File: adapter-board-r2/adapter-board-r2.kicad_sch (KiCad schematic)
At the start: 47 parts, among them J1 USB_C_Receptacle_USB2.0_14P, J2 Conn_01x02_Socket, J3 Conn_01x04_Socket, J4 Conn_01x07_Pin, Q1 UMH3N, Q2 BSS138W, Q3 BSS138W, U1 ESP32-C3-WROOM-02, U2 USBLC6-2SC6, U3 CH340X, U4 AP2114HA-3.3TRG1, U5 ENS210, U6 LIS2DW12TR, U7 SCD40-D-R2, U8 YSN8900AP3, U9 BMP580

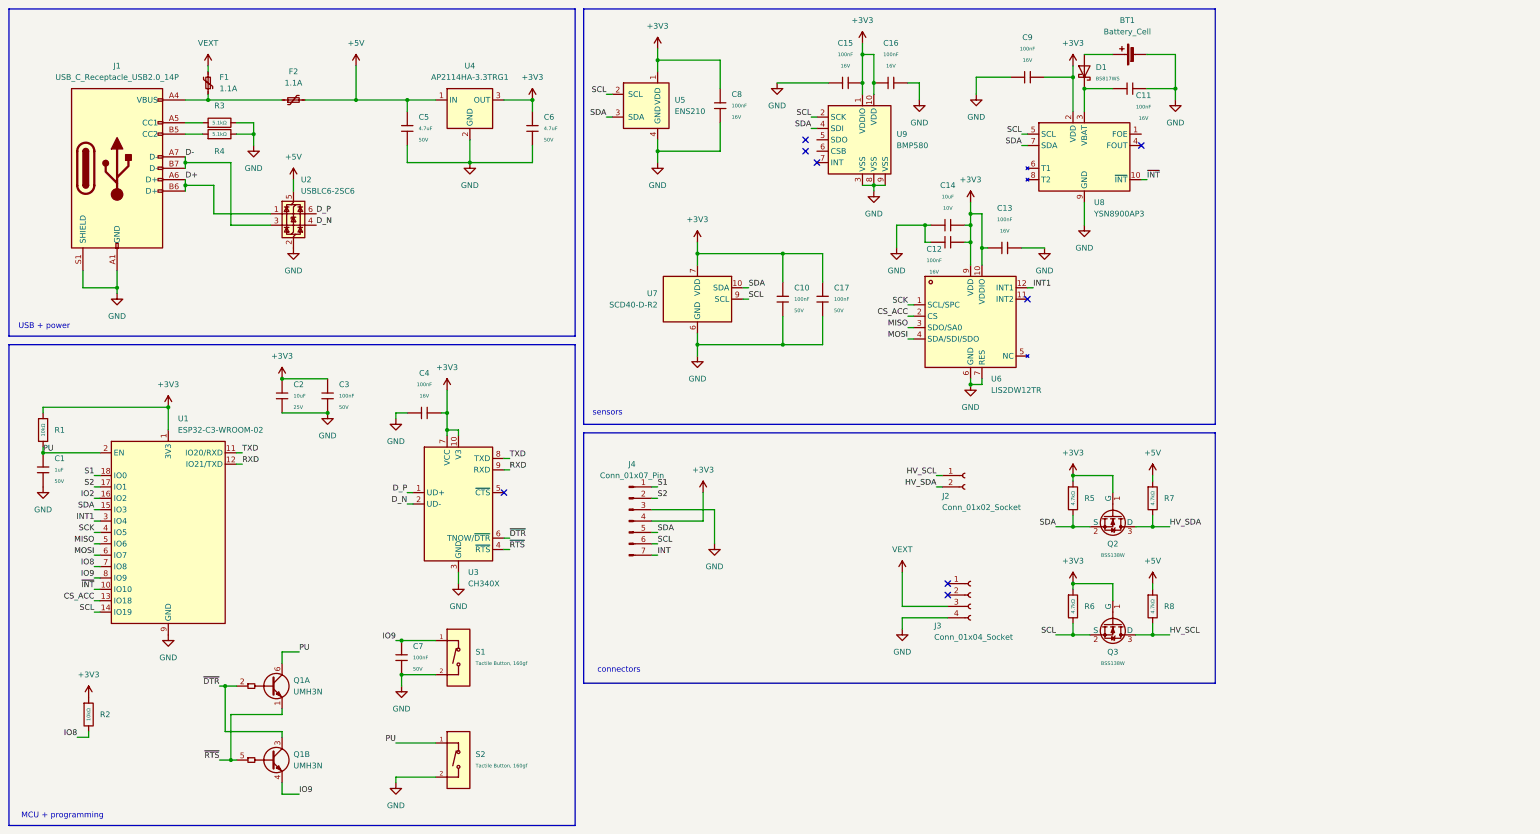
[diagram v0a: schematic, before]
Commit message: feat: updated pcb
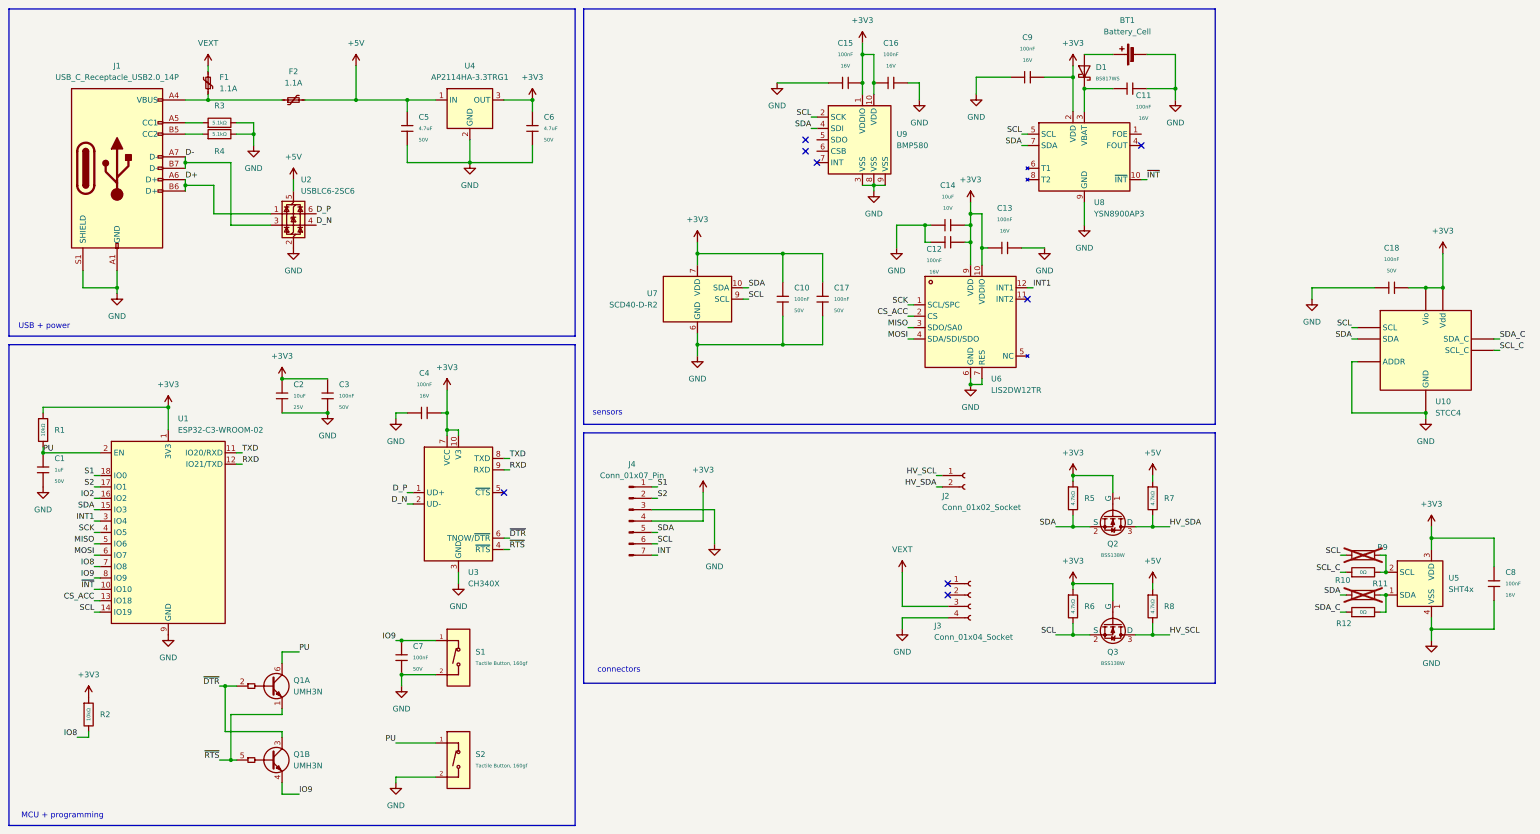
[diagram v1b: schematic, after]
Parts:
- removed U5: ENS210, Package_DFN_QFN:AMS_QFN-4-1EP_2x2mm_P0.95mm_EP0.7x1.6mm, symbol Sensor_Humidity:ENS210
- added C18: 100nF, PCM_JLCPCB:C_0603, symbol PCM_JLCPCB-Capacitors:0603,100nF
- added R10, R11, R12, R9: 0Ω, PCM_JLCPCB:R_0402, symbol PCM_JLCPCB-Resistors:0402,0Ω
- added U10: STCC4, custom:STCC4, symbol custom:STCC4
- added U5: SHT4x, Sensor_Humidity:Sensirion_DFN-4_1.5x1.5mm_P0.8mm_SHT4x_NoCentralPad, symbol Sensor_Humidity:SHT4x
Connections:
- net +3V3: now also C18.2, U10.6 (Vio), U10.7 (Vdd), U5.3 (VDD)
- net GND: now also C18.1, U10.3 (ADDR), U10.4 (GND), U5.4 (VSS)
- net SCL: now also R9.1, U10.1 (SCL)
- net SDA: now also R11.1, U10.5 (SDA)
- new net: R11.2, R12.2, U5.1 (SDA)
- new net: R10.2, R9.2, U5.2 (SCL)
- new net SCL_C: R10.1, U10.8 (SCL_C)
- new net SDA_C: R12.1, U10.2 (SDA_C)
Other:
- moved on the sheet: C8
